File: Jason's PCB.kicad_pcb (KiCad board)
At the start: 2 copper layers, 66.7 x 85.7 mm, 11 parts, among them U1 Elite-C

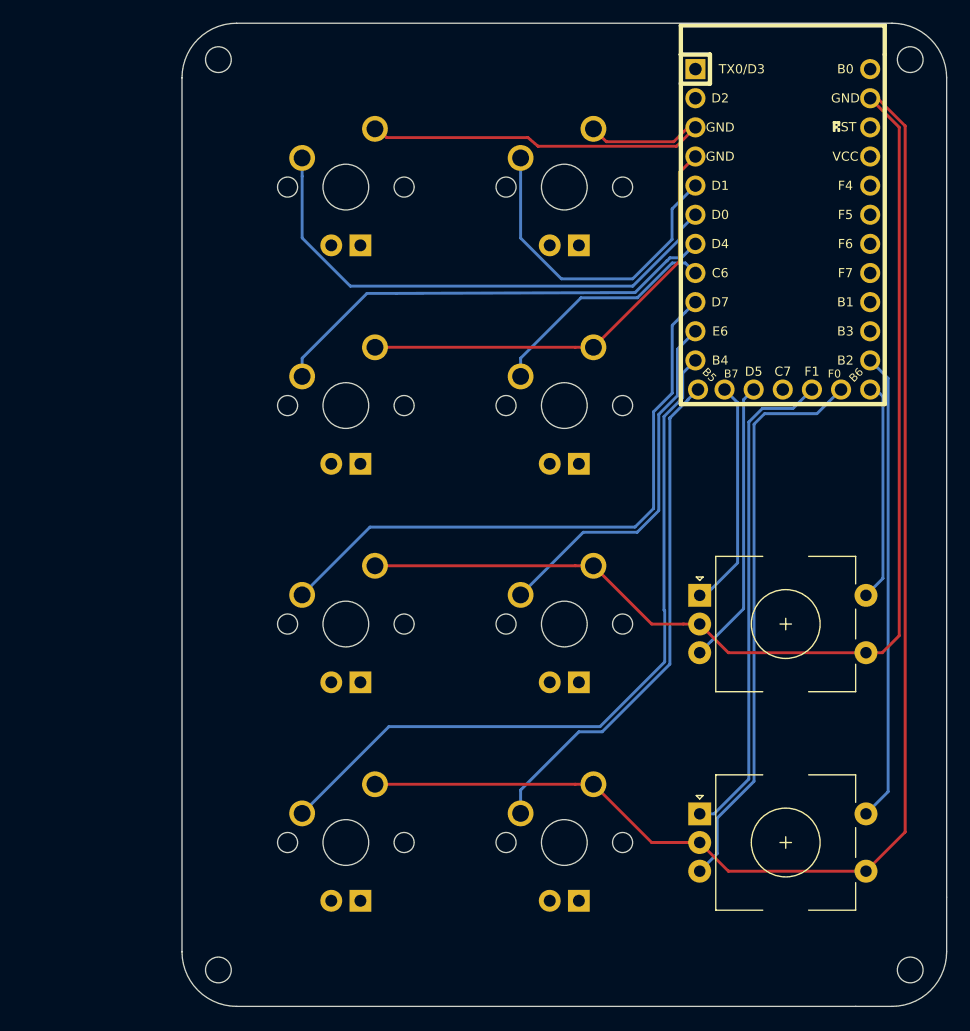
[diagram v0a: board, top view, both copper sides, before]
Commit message: More routing changes
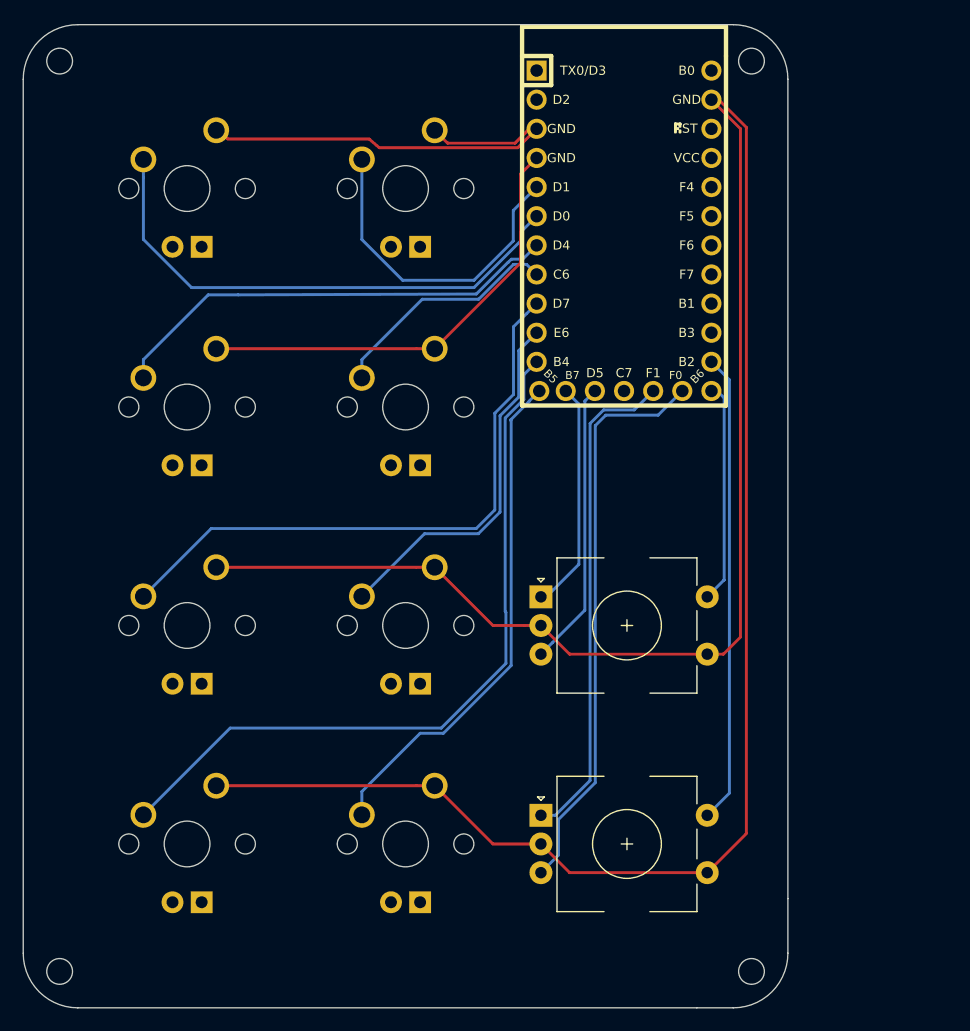
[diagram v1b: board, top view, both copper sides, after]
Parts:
- moved U1 13.8 mm to (138.6, 38.7)
- moved SW_A1 13.8 mm to (100.5, 35.1)
- moved SW_B1 13.8 mm to (100.5, 54.1)
- moved SW_C1 13.8 mm to (100.5, 73.2)
- moved SW_D1 13.8 mm to (100.5, 92.2)
- moved SW_A2 13.8 mm to (119.5, 35.1)
- moved SW_B2 13.8 mm to (119.5, 54.1)
- moved SW_C2 13.8 mm to (119.5, 73.2)
- moved SW_D2 13.8 mm to (119.5, 92.2)
- moved SW_E1 13.8 mm to (138.8, 73.2)
- moved SW_E2 13.8 mm to (138.8, 92.2)
